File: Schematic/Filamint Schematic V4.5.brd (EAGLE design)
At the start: 102.5 x 69.8 mm, 31 parts, among them IC1 7805DT, U1 ATMEGA328P_PDIP

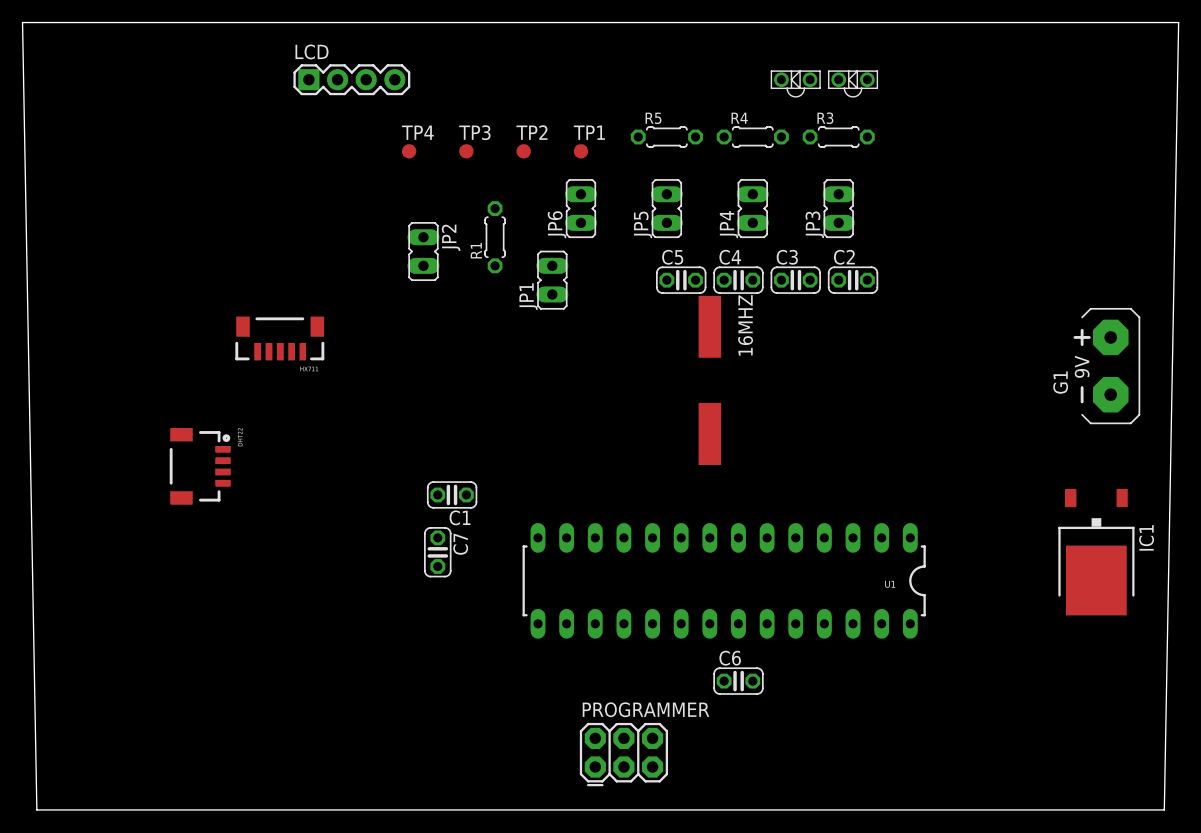
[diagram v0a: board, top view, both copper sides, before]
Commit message: very*very* rough draft
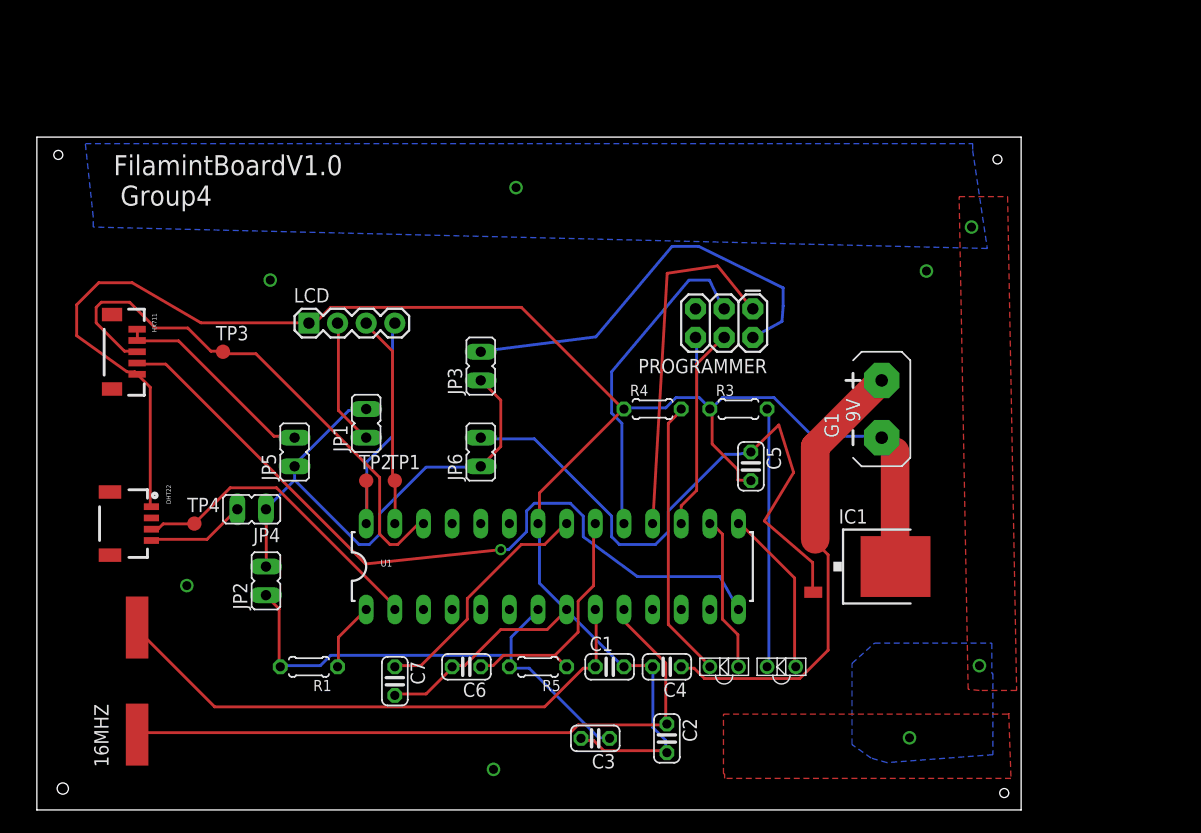
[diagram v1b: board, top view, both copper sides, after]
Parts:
- moved 16MHZ 57.4 mm to (8.89, 11.4), turned to 90 degrees
- moved LED1 52.5 mm to (66.0, 12.7)
- moved LED2 52.5 mm to (61.0, 12.7)
- moved JP4 51.8 mm to (19.1, 26.7), turned to 90 degrees
- moved R5 48.4 mm to (44.5, 12.7), turned to 180 degrees
- moved C3 44.4 mm to (49.5, 6.35), turned to 180 degrees
- moved C2 43.9 mm to (55.9, 6.35), turned to 270 degrees
- moved PROGRAMMER 43.0 mm to (63.5, 44.5), turned to 180 degrees
- moved R1 41.5 mm to (24.1, 12.7), turned to 180 degrees
- moved JP5 39.5 mm to (22.9, 31.8)
- moved TP4 38.1 mm to (14.0, 25.4)
- moved C4 34.9 mm to (55.9, 12.7), turned to 180 degrees
- moved JP3 34.7 mm to (39.4, 39.4)
- moved TP1 33.6 mm to (31.8, 29.2)
- moved JP2 32.4 mm to (20.3, 20.3), turned to 0 degrees
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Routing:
- net GND: track 0.00 -> 194.2 mm
- net CLK: track 0.00 -> 68.8 mm, vias 0 -> 1
- net N$2: track 0.00 -> 59.2 mm
- net N$29: track 0.00 -> 54.5 mm
- net VCC: track 0.00 -> 50.4 mm
- net N$1: track 0.00 -> 50.2 mm
- net WGHT_SIG: track 0.00 -> 47.9 mm
- net N$27: track 0.00 -> 45.4 mm
- net VIN: track 0.00 -> 41.6 mm
- net N$26: track 0.00 -> 37.4 mm
- net N$7: track 0.00 -> 32.0 mm
- net N$6: track 0.00 -> 29.2 mm
- net HUM_SIG: track 0.00 -> 27.8 mm
- net N$25: track 0.00 -> 24.9 mm
- net N$24: track 0.00 -> 23.2 mm
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- added copper zone on layer 1, net GND
- added copper zone on layer 16, net GND
- added copper zone on layer 1, net N$17
- added copper zone on layer 16, net N$19
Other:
- board size 102.5 x 69.8 mm -> 87.3 x 59.7 mm
- board text added: "FilamintBoardV1.0"
- board text added: "Group4"
